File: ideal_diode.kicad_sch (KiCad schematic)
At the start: 11 parts, among them Q3 NVMFS5C404NL, U10 SN74LVC2G08, U11 LM74700

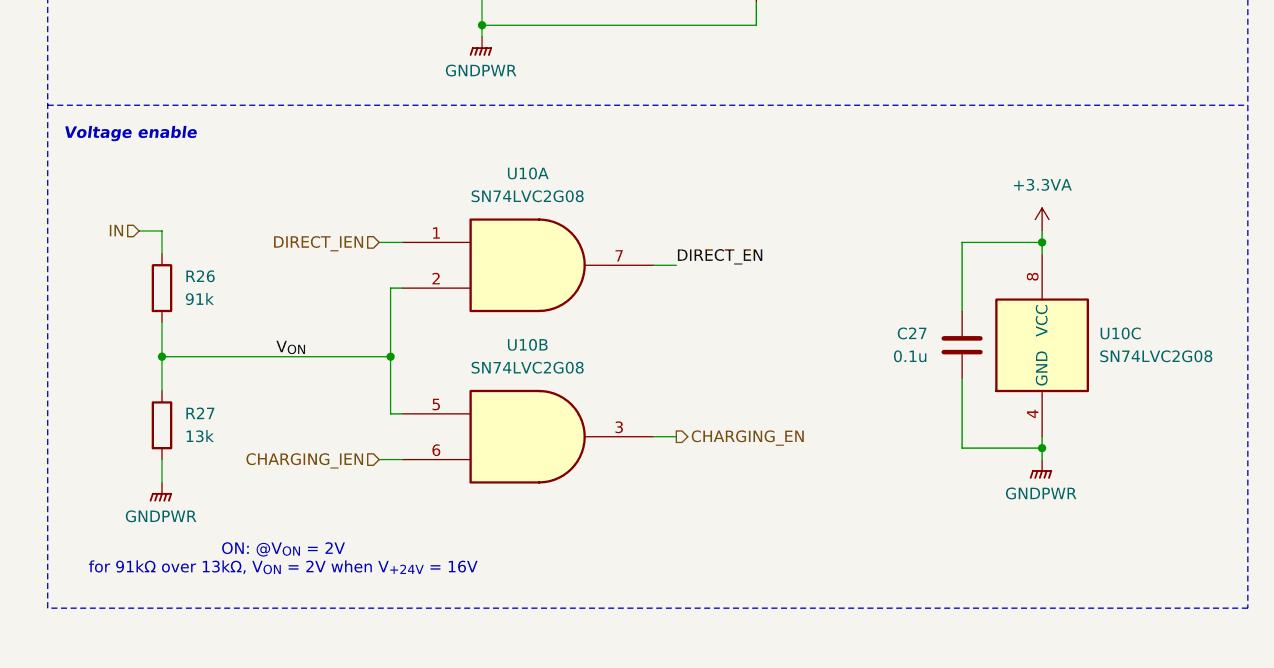
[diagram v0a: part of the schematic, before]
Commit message: Ideating for diff amp
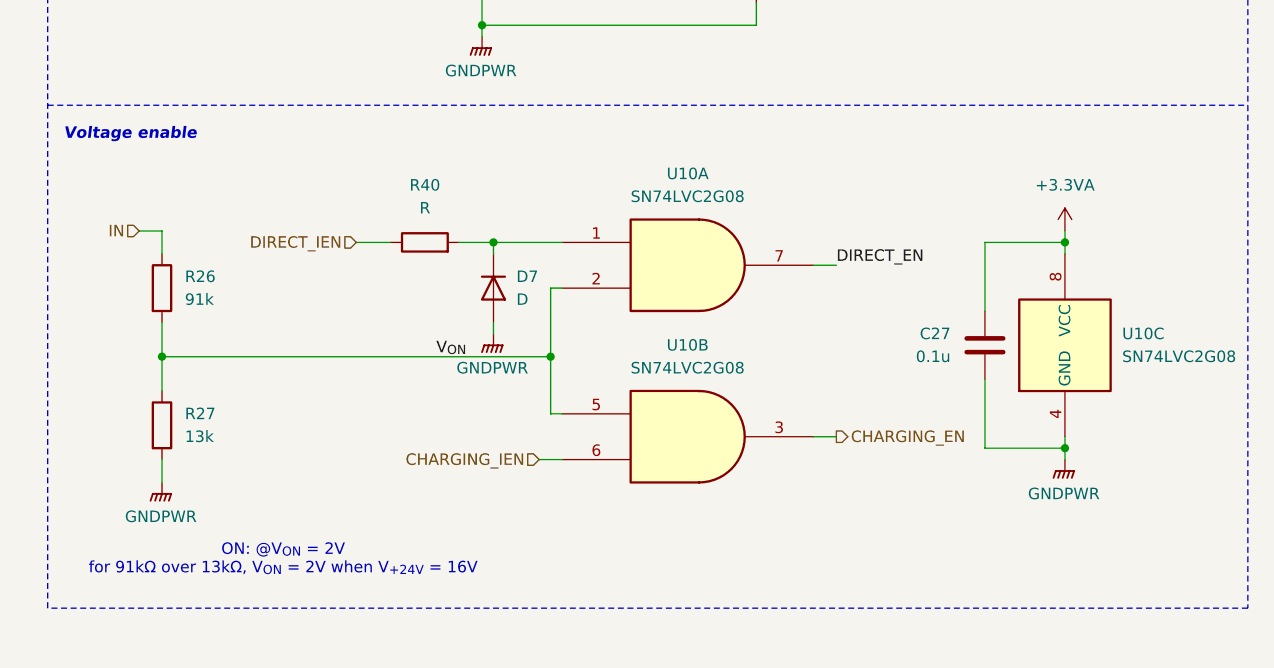
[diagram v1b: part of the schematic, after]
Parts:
- added D7: D, symbol Device:D
- added R40: R, symbol Device:R
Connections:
- net DIRECT_IEN: now also R40.1; no longer U10.1
- net GNDPWR: now also D7.2 (A)
- new net: D7.1 (K), R40.2, U10.1
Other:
- moved on the sheet: C27, U10A, U10B, U10C
